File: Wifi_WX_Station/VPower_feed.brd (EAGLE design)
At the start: 34 x 37.5 mm, 5 parts, among them J1 RJ45-8VERT, J2 RJ45-8VERT

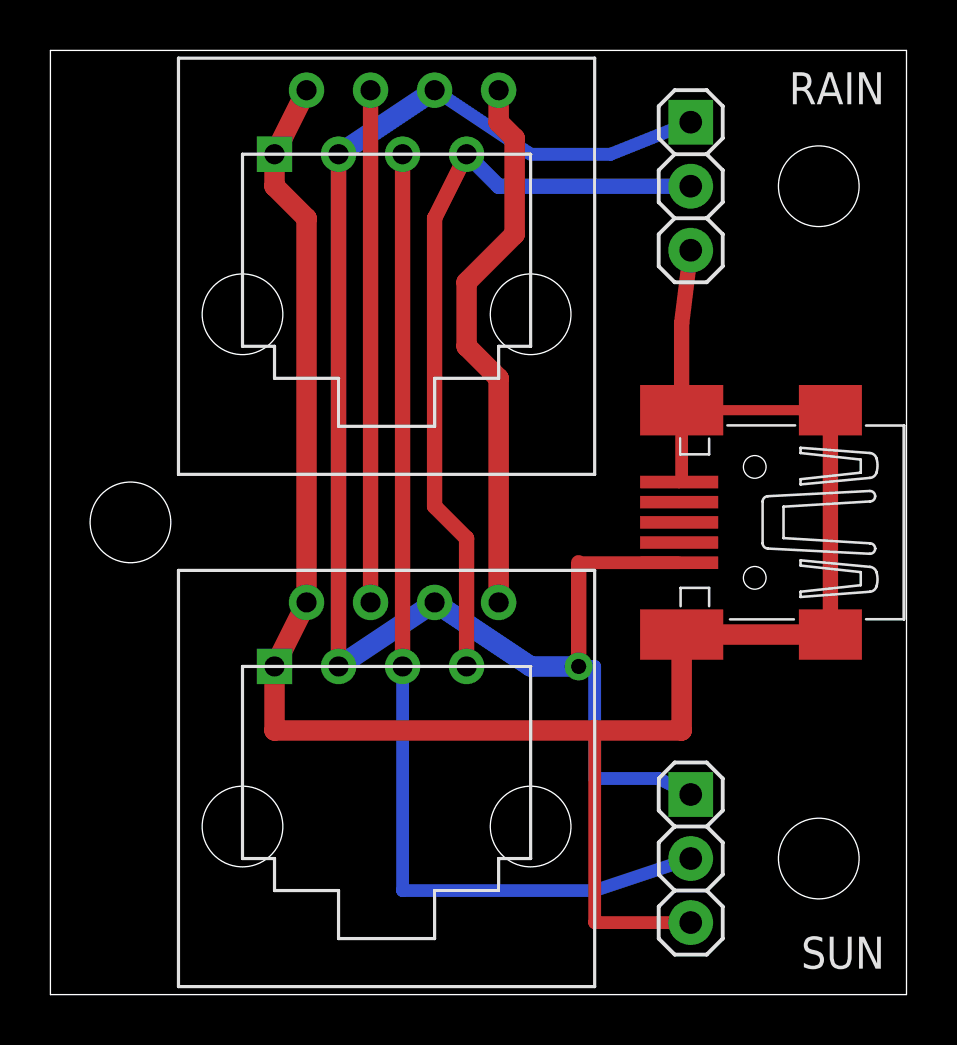
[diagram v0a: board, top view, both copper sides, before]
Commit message: updated BOM with all prices- As Checked in to BATCH PCB
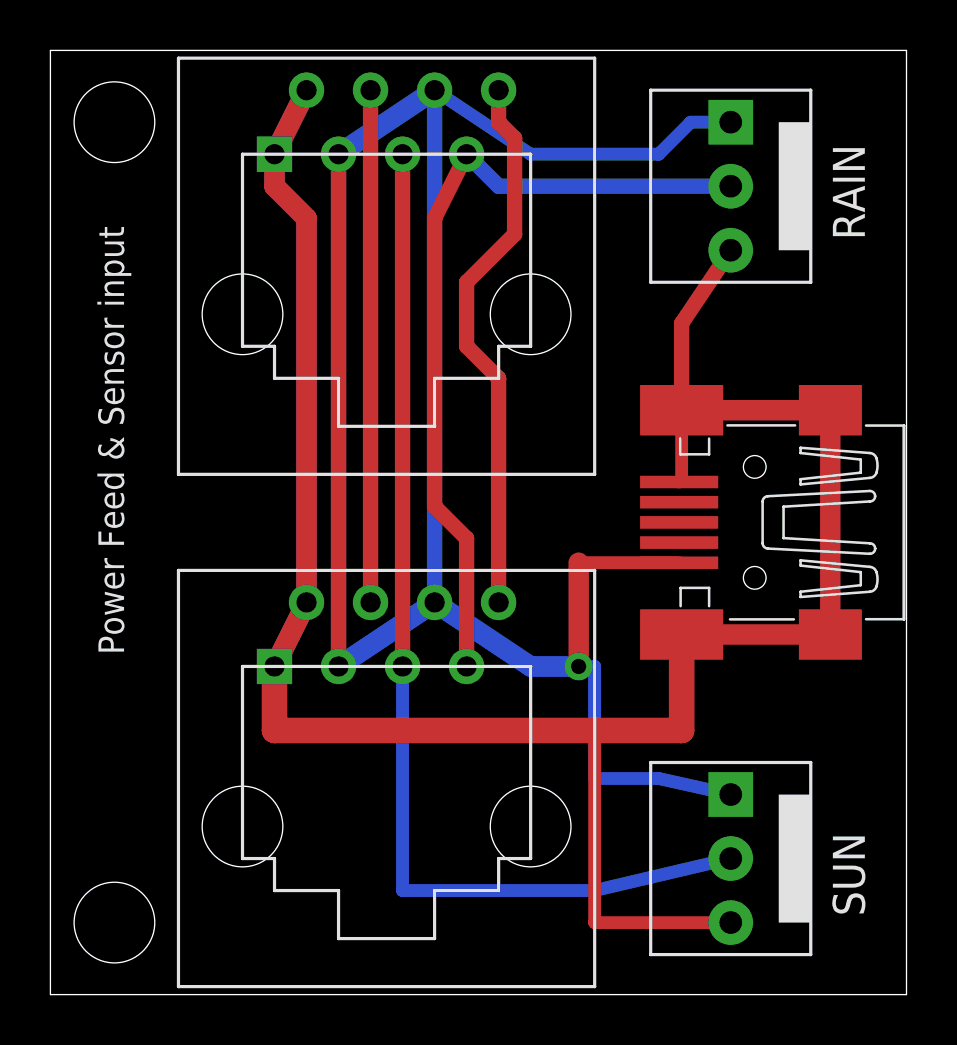
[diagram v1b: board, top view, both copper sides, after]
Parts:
- RAIN, SUN: device wifi_WX:1X03 -> wifi_WX:1X3_MOLEX_KK
- moved SUN 4.13 mm to (28.9, 12.7)
- moved RAIN 4.13 mm to (28.9, 39.4)
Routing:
- net GND: track 87.9 -> 114.0 mm
- net +5V: track 85.7 -> 109.4 mm
- net RAIN_CNT_IN: track 30.6 -> 32.1 mm
- net SUN_IN: track 40.8 -> 42.4 mm
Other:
- board text added: "Power Feed & Sensor input"
- board text removed: "WX Power Feed"
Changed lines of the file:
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@@
 <wire x1="39.04" y1="40.9475" x2="5.08" y2="40.9475" width="0" layer="20"/>
 <wire x1="5.08" y1="40.9475" x2="5.08" y2="3.4925" width="0" layer="20"/>
-<hole x="35.56" y="8.89" drill="3.2"/>
-<hole x="35.56" y="35.56" drill="3.2"/>
-<hole x="8.255" y="22.225" drill="3.2"/>
-<text x="36.83" y="32.385" size="1.27" layer="22" rot="MR270">RV-Builders Products 2013</text>
-<text x="31.75" y="29.21" size="1.27" layer="22" rot="MR270">WX Power Feed </text>
+<hole x="7.62" y="6.35" drill="3.2"/>
+<hole x="7.62" y="38.1" drill="3.2"/>
+<text x="36.83" y="36.195" size="1.27" layer="22" font="vector" rot="MR270">RV-Builders Products 2013</text>
+<text x="6.985" y="33.9725" size="1.016" layer="21" font="vector" rot="R270">Power Feed &amp; Sensor input</text>
 </plain>
 <attributes>
@@
 <element name="J2" library="wifi_WX" package="RJ45_VERT" value="RJ45-8VERT" x="12.7" y="10.16"/>
 <element name="USB" library="wifi_WX" package="32005-301" value="MINI-USB-32005-301" x="33.02" y="22.225" smashed="yes" rot="R180"/>
-<element name="RAIN" library="wifi_WX" package="1X03" value="" x="30.48" y="35.56" smashed="yes" rot="R270">
-<attribute name="NAME" x="38.1762" y="40.0812" size="1.27" layer="25" ratio="10" rot="R180"/>
-<attribute name="VALUE" x="27.305" y="39.37" size="1.27" layer="27" rot="R270"/>
+<element name="RAIN" library="wifi_WX" package="1X3_MOLEX_KK" value="" x="28.8925" y="39.37" smashed="yes" rot="R270">
+<attribute name="NAME" x="36.1188" y="37.2237" size="1.27" layer="25" font="vector" ratio="10" rot="R270"/>
+<attribute name="VALUE" x="25.7175" y="43.18" size="1.27" layer="27" rot="R270"/>
 </element>
-<element name="SUN" library="wifi_WX" package="1X03" value="" x="30.48" y="8.89" smashed="yes" rot="R270">
-<attribute name="NAME" x="38.1762" y="5.7912" size="1.27" layer="25" ratio="10" rot="R180"/>
-<attribute name="VALUE" x="27.305" y="12.7" size="1.27" layer="27" rot="R270"/>
+<element name="SUN" library="wifi_WX" package="1X3_MOLEX_KK" value="" x="28.8925" y="12.7" smashed="yes" rot="R270">
+<attribute name="NAME" x="36.1188" y="9.9187" size="1.27" layer="25" font="vector" ratio="10" rot="R270"/>
+<attribute name="VALUE" x="25.7175" y="16.51" size="1.27" layer="27" rot="R270"/>
 </element>
 </elements>
@@
 <contactref element="USB" pad="M1"/>
 <contactref element="RAIN" pad="3"/>
-<wire x1="36.02" y1="26.675" x2="30.12" y2="26.675" width="0.4064" layer="1"/>
+<wire x1="36.02" y1="26.675" x2="30.12" y2="26.675" width="0.8128" layer="1"/>
 <wire x1="30.12" y1="17.775" x2="36.02" y2="17.775" width="0.8128" layer="1"/>
 <wire x1="15.24" y1="39.37" x2="13.97" y2="36.83" width="0.8128" layer="1"/>
-<wire x1="30.12" y1="13.97" x2="30.12" y2="17.775" width="0.8128" layer="1"/>
+<wire x1="30.12" y1="13.97" x2="30.12" y2="17.775" width="1.016" layer="1"/>
 <wire x1="15.24" y1="19.05" x2="15.24" y2="34.29" width="0.8128" layer="1"/>
 <wire x1="15.24" y1="34.29" x2="13.97" y2="35.56" width="0.8128" layer="1"/>
 <wire x1="13.97" y1="35.56" x2="13.97" y2="36.83" width="0.8128" layer="1"/>
 <wire x1="15.24" y1="19.05" x2="13.97" y2="16.51" width="0.8128" layer="1"/>
-<wire x1="13.97" y1="16.51" x2="13.97" y2="13.97" width="0.8128" layer="1"/>
-<wire x1="13.97" y1="13.97" x2="26.67" y2="13.97" width="0.8128" layer="1"/>
-<wire x1="26.67" y1="13.97" x2="30.12" y2="13.97" width="0.8128" layer="1"/>
-<wire x1="36.02" y1="17.775" x2="36.02" y2="26.675" width="0.6096" layer="1"/>
-<wire x1="30.48" y1="33.02" x2="30.12" y2="30.12" width="0.6096" layer="1"/>
+<wire x1="13.97" y1="16.51" x2="13.97" y2="13.97" width="1.016" layer="1"/>
+<wire x1="13.97" y1="13.97" x2="26.67" y2="13.97" width="1.016" layer="1"/>
+<wire x1="26.67" y1="13.97" x2="30.12" y2="13.97" width="1.016" layer="1"/>
+<wire x1="36.02" y1="17.775" x2="36.02" y2="26.675" width="0.8128" layer="1"/>
+<wire x1="32.0675" y1="33.02" x2="30.12" y2="30.12" width="0.6096" layer="1"/>
 <wire x1="30.12" y1="30.12" x2="30.12" y2="26.675" width="0.6096" layer="1"/>
 <wire x1="30.02" y1="23.825" x2="30.12" y2="23.925" width="0.508" layer="1"/>
 <wire x1="30.12" y1="23.925" x2="30.12" y2="26.675" width="0.508" layer="1"/>
 <contactref element="SUN" pad="3"/>
-<wire x1="30.48" y1="6.35" x2="26.67" y2="6.35" width="0.508" layer="1"/>
+<wire x1="32.0675" y1="6.35" x2="26.67" y2="6.35" width="0.508" layer="1"/>
 <wire x1="26.67" y1="6.35" x2="26.67" y2="13.97" width="0.508" layer="1"/>
+<wire x1="13.97" y1="16.51" x2="15.24" y2="19.05" width="0.8128" layer="16"/>
+<wire x1="15.24" y1="19.05" x2="15.24" y2="34.29" width="0.8128" layer="16"/>
+<wire x1="15.24" y1="34.29" x2="13.97" y2="35.56" width="0.8128" layer="16"/>
+<wire x1="13.97" y1="35.56" x2="13.97" y2="36.83" width="0.8128" layer="16"/>
+<wire x1="13.97" y1="36.83" x2="15.24" y2="39.37" width="0.8128" layer="16"/>
 </signal>
 <signal name="+5V">
@@
 <wire x1="16.51" y1="36.83" x2="16.51" y2="16.51" width="0.6096" layer="16"/>
 <wire x1="30.02" y1="20.625" x2="26.035" y2="20.625" width="0.508" layer="1"/>
-<wire x1="26.035" y1="20.625" x2="26.035" y2="16.51" width="0.6096" layer="1"/>
+<wire x1="26.035" y1="20.625" x2="26.035" y2="16.51" width="0.8128" layer="1"/>
 <wire x1="20.32" y1="39.37" x2="24.13" y2="36.83" width="0.508" layer="16"/>
-<wire x1="24.13" y1="36.83" x2="27.305" y2="36.83" width="0.508" layer="16"/>
-<wire x1="27.305" y1="36.83" x2="30.48" y2="38.1" width="0.508" layer="16"/>
+<wire x1="24.13" y1="36.83" x2="29.21" y2="36.83" width="0.508" layer="16"/>
 <contactref element="SUN" pad="1"/>
 <wire x1="26.035" y1="16.51" x2="26.67" y2="16.51" width="0.508" layer="16"/>
 <wire x1="26.67" y1="16.51" x2="26.67" y2="12.065" width="0.508" layer="16"/>
 <wire x1="26.67" y1="12.065" x2="29.21" y2="12.065" width="0.508" layer="16"/>
-<wire x1="29.21" y1="12.065" x2="30.48" y2="11.43" width="0.508" layer="16"/>
+<wire x1="29.21" y1="12.065" x2="32.0675" y2="11.43" width="0.508" layer="16"/>
+<wire x1="29.21" y1="36.83" x2="30.48" y2="38.1" width="0.508" layer="16"/>
+<wire x1="30.48" y1="38.1" x2="32.0675" y2="38.1" width="0.508" layer="16"/>
+<wire x1="20.32" y1="39.37" x2="20.32" y2="19.05" width="0.6096" layer="16"/>
 </signal>
 <signal name="WIN_DIR_IN">
@@
 <wire x1="19.05" y1="16.51" x2="19.05" y2="7.62" width="0.508" layer="16"/>
 <wire x1="19.05" y1="7.62" x2="26.67" y2="7.62" width="0.508" layer="16"/>
-<wire x1="26.67" y1="7.62" x2="30.48" y2="8.89" width="0.508" layer="16"/>
+<wire x1="26.67" y1="7.62" x2="32.0675" y2="8.89" width="0.508" layer="16"/>
 </signal>
 <signal name="RAIN_CNT_IN">
@@
 <wire x1="20.32" y1="22.86" x2="21.59" y2="21.59" width="0.6096" layer="1"/>
 <wire x1="21.59" y1="21.59" x2="21.59" y2="16.51" width="0.6096" layer="1"/>
-<wire x1="30.48" y1="35.56" x2="22.86" y2="35.56" width="0.6096" layer="16"/>
+<wire x1="32.0675" y1="35.56" x2="22.86" y2="35.56" width="0.6096" layer="16"/>
 <wire x1="22.86" y1="35.56" x2="22.86" y2="34.925" width="0" layer="19" extent="1-16"/>
 <wire x1="22.86" y1="35.56" x2="21.59" y2="36.83" width="0.6096" layer="16"/>
@@
 <contactref element="J1" pad="P$8"/>
 <contactref element="J2" pad="P$8"/>
-<wire x1="22.86" y1="39.37" x2="22.86" y2="38.1" width="0.8128" layer="1"/>
-<wire x1="22.86" y1="38.1" x2="23.495" y2="37.465" width="0.8128" layer="1"/>
-<wire x1="23.495" y1="37.465" x2="23.495" y2="33.655" width="0.8128" layer="1"/>
-<wire x1="23.495" y1="33.655" x2="21.59" y2="31.75" width="0.8128" layer="1"/>
-<wire x1="21.59" y1="31.75" x2="21.59" y2="29.21" width="0.8128" layer="1"/>
-<wire x1="21.59" y1="29.21" x2="22.86" y2="27.94" width="0.8128" layer="1"/>
-<wire x1="22.86" y1="27.94" x2="22.86" y2="19.05" width="0.8128" layer="1"/>
+<wire x1="22.86" y1="39.37" x2="22.86" y2="38.1" width="0.6096" layer="1"/>
+<wire x1="22.86" y1="38.1" x2="23.495" y2="37.465" width="0.6096" layer="1"/>
+<wire x1="23.495" y1="37.465" x2="23.495" y2="33.655" width="0.6096" layer="1"/>
+<wire x1="23.495" y1="33.655" x2="21.59" y2="31.75" width="0.6096" layer="1"/>
+<wire x1="21.59" y1="31.75" x2="21.59" y2="29.21" width="0.6096" layer="1"/>
+<wire x1="21.59" y1="29.21" x2="22.86" y2="27.94" width="0.6096" layer="1"/>
+<wire x1="22.86" y1="27.94" x2="22.86" y2="19.05" width="0.6096" layer="1"/>
 </signal>
 </signals>
